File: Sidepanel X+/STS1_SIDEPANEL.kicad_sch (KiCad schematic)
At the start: 3 parts, among them J1 Conn_02x04_Odd_Even, J2 Conn_02x02_Odd_Even

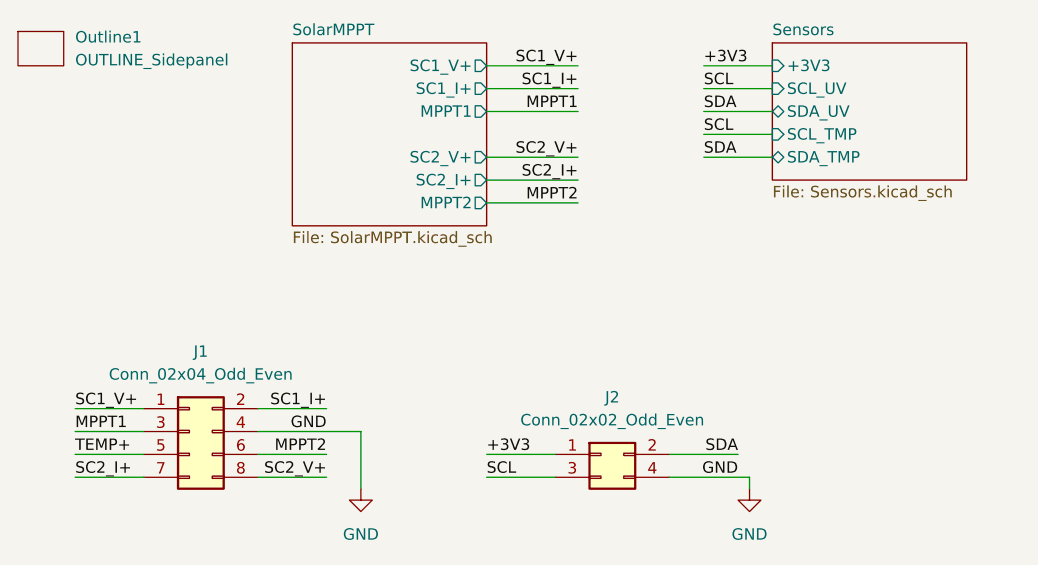
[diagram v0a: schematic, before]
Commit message: Review Ready for V2.0
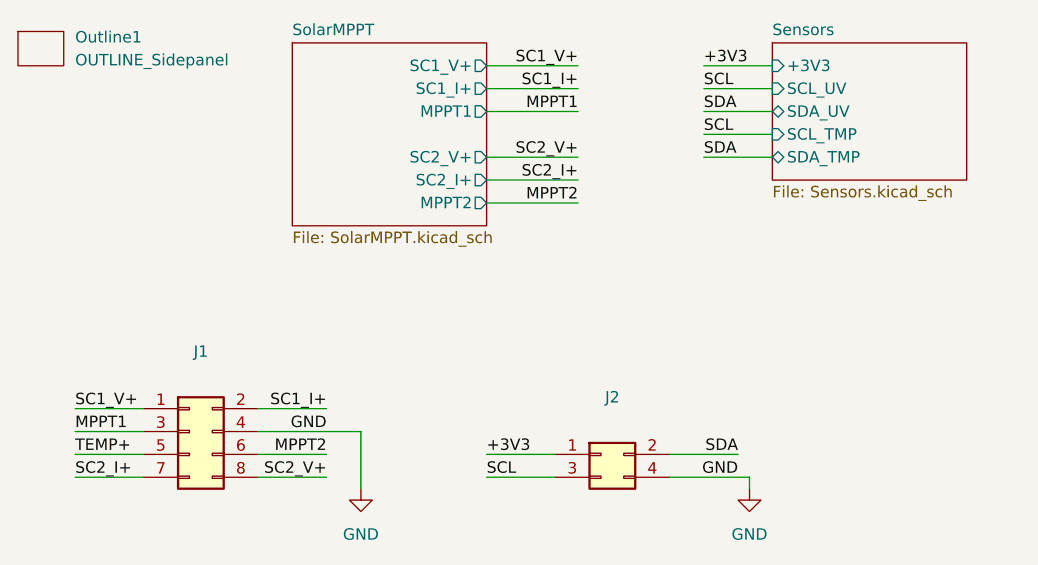
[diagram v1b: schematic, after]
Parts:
- J1: value Conn_02x04_Odd_Even -> (none); footprint SamacSys:M808280842 -> (none)
- J2: value Conn_02x02_Odd_Even -> (none); footprint USER_Passiv:M80-8280442 -> (none)
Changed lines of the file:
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@@
     (in_bom yes) (on_board yes) (fields_autoplaced)
     (property "Reference" "J1" (id 0) (at 40.64 60.96 0))
-    (property "Value" "Conn_02x04_Odd_Even" (id 1) (at 40.64 63.5 0))
-    (property "Footprint" "SamacSys:M808280842" (id 2) (at 39.37 69.85 0)
+    (property "Value" "" (id 1) (at 40.64 63.5 0))
+    (property "Footprint" "" (id 2) (at 39.37 69.85 0)
       (effects (font (size 1.27 1.27)) hide)
     )
@@
     (in_bom yes) (on_board yes) (fields_autoplaced)
     (property "Reference" "J2" (id 0) (at 86.36 66.04 0))
-    (property "Value" "Conn_02x02_Odd_Even" (id 1) (at 86.36 68.58 0))
-    (property "Footprint" "USER_Passiv:M80-8280442" (id 2) (at 85.09 72.39 0)
+    (property "Value" "" (id 1) (at 86.36 68.58 0))
+    (property "Footprint" "" (id 2) (at 85.09 72.39 0)
       (effects (font (size 1.27 1.27)) hide)
     )
@@
     )
     (path "/4f87559b-6bba-4ff6-97a7-dad9a308db2d/934b6342-5d8d-49da-bf4f-f7fa77f16f34"
-      (reference "CUR1") (unit 1) (value "TMCS1101A3BQDT") (footprint "SOIC127P600X175-8N")
+      (reference "CUR1") (unit 1) (value "TMCS1101A3BQDT") (footprint "Package_SO:SOIC-8_3.9x4.9mm_P1.27mm")
     )
     (path "/4f87559b-6bba-4ff6-97a7-dad9a308db2d/a554cf31-0806-4740-ba0b-f0d59599f4ca"
@@
     )
     (path "/4f87559b-6bba-4ff6-97a7-dad9a308db2d/c6a198d2-e0e4-4d6d-8a2a-bdeb249501be"
-      (reference "DOUT1") (unit 1) (value "SMM4F5.0") (footprint "SamacSys:STMITE")
+      (reference "DOUT1") (unit 1) (value "SMM4F5.0") (footprint "Diode_SMD:D_0603_1608Metric")
     )
     (path "/9d03bb93-a9aa-424f-bd25-022f173efd1d/d9839939-8918-48f3-b4b2-d753b1d9a645"
-      (reference "IC1") (unit 1) (value "TMP112AQDRLRQ1") (footprint "SamacSys:SOTFL50P160X60-6N")
+      (reference "IC1") (unit 1) (value "TMP112AQDRLRQ1") (footprint "Package_TO_SOT_SMD:SOT-563")
     )
     (path "/7d4ab197-adca-450c-9fc5-7a95ff72b885"
-      (reference "J1") (unit 1) (value "Conn_02x04_Odd_Even") (footprint "SamacSys:M808280842")
+      (reference "J1") (unit 1) (value "Conn_02x04_Odd_Even") (footprint "STS_Connector:M808280842")
     )
     (path "/9272ccd5-e950-4f99-baec-47da7f19129b"
-      (reference "J2") (unit 1) (value "Conn_02x02_Odd_Even") (footprint "USER_Passiv:M80-8280442")
+      (reference "J2") (unit 1) (value "Conn_02x02_Odd_Even") (footprint "STS_Connector:M808280442")
     )
     (path "/4f87559b-6bba-4ff6-97a7-dad9a308db2d/bfe4e68f-4cef-4b31-adff-8df094bc3870"
-      (reference "L_IN1") (unit 1) (value "10u") (footprint "SamacSys:INDPM5650X530N")
+      (reference "L_IN1") (unit 1) (value "10u") (footprint "Inductor_SMD:L_0805_2012Metric")
     )
     (path "/4f87559b-6bba-4ff6-97a7-dad9a308db2d/679b2e27-da22-4f13-a86e-25be83598a10"
-      (reference "MPPT1") (unit 1) (value "SPV1040TTR") (footprint "SamacSys:SOP65P640X120-8N")
+      (reference "MPPT1") (unit 1) (value "SPV1040TTR") (footprint "Package_SO:TSSOP-8_4.4x3mm_P0.65mm")
     )
     (path "/6503b427-07c6-4391-8fa6-4757fb4daa6c"
@@
     )
     (path "/4f87559b-6bba-4ff6-97a7-dad9a308db2d/e7b54c2f-482e-4a97-841f-62a80e0193a8"
-      (reference "SC1") (unit 1) (value "Solar_Cell") (footprint "USER_Activ:3G30A_40x80")
+      (reference "SC1") (unit 1) (value "Solar_Cell") (footprint "STS_Connector:3G30A_40x80")
     )
     (path "/9d03bb93-a9aa-424f-bd25-022f173efd1d/a83d6342-0e16-4131-8bb9-e65e4d72dab0"
-      (reference "U1") (unit 1) (value "GUVA-C32SM") (footprint "USER_Optic:OLGA 2mm x 2,3mm")
-    )
-  )
+      (reference "U1") (unit 1) (value "GUVA-C32SM") (footprint "Package_SO:SO-4_4.4x3.6mm_P2.54mm")
+    )
+  )

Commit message: Further fixes, still some open
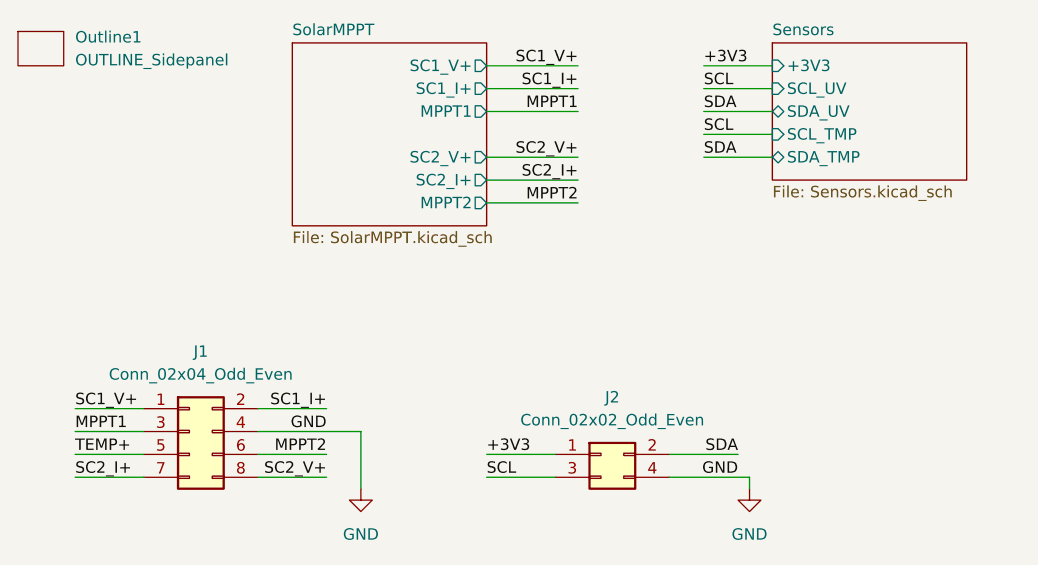
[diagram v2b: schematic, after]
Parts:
- J1: value (none) -> Conn_02x04_Odd_Even; footprint (none) -> STS_Connector:M808280842
- J2: value (none) -> Conn_02x02_Odd_Even; footprint (none) -> STS_Connector:M808280442
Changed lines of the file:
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@@
     (in_bom yes) (on_board yes) (fields_autoplaced)
     (property "Reference" "J1" (id 0) (at 40.64 60.96 0))
-    (property "Value" "" (id 1) (at 40.64 63.5 0))
-    (property "Footprint" "" (id 2) (at 39.37 69.85 0)
+    (property "Value" "Conn_02x04_Odd_Even" (id 1) (at 40.64 63.5 0))
+    (property "Footprint" "STS_Connector:M808280842" (id 2) (at 39.37 69.85 0)
       (effects (font (size 1.27 1.27)) hide)
     )
@@
     (in_bom yes) (on_board yes) (fields_autoplaced)
     (property "Reference" "J2" (id 0) (at 86.36 66.04 0))
-    (property "Value" "" (id 1) (at 86.36 68.58 0))
-    (property "Footprint" "" (id 2) (at 85.09 72.39 0)
+    (property "Value" "Conn_02x02_Odd_Even" (id 1) (at 86.36 68.58 0))
+    (property "Footprint" "STS_Connector:M808280442" (id 2) (at 85.09 72.39 0)
       (effects (font (size 1.27 1.27)) hide)
     )
